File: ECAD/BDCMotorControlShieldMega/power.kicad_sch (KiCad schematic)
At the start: 23 parts, among them Q1 Q_PMOS, Q2 Q_PMOS, Q3 Q_NMOS, Q4 Q_NMOS, Q5 Q_PNP, Q6 Q_PNP, U14 LMV331, U33 LM2776

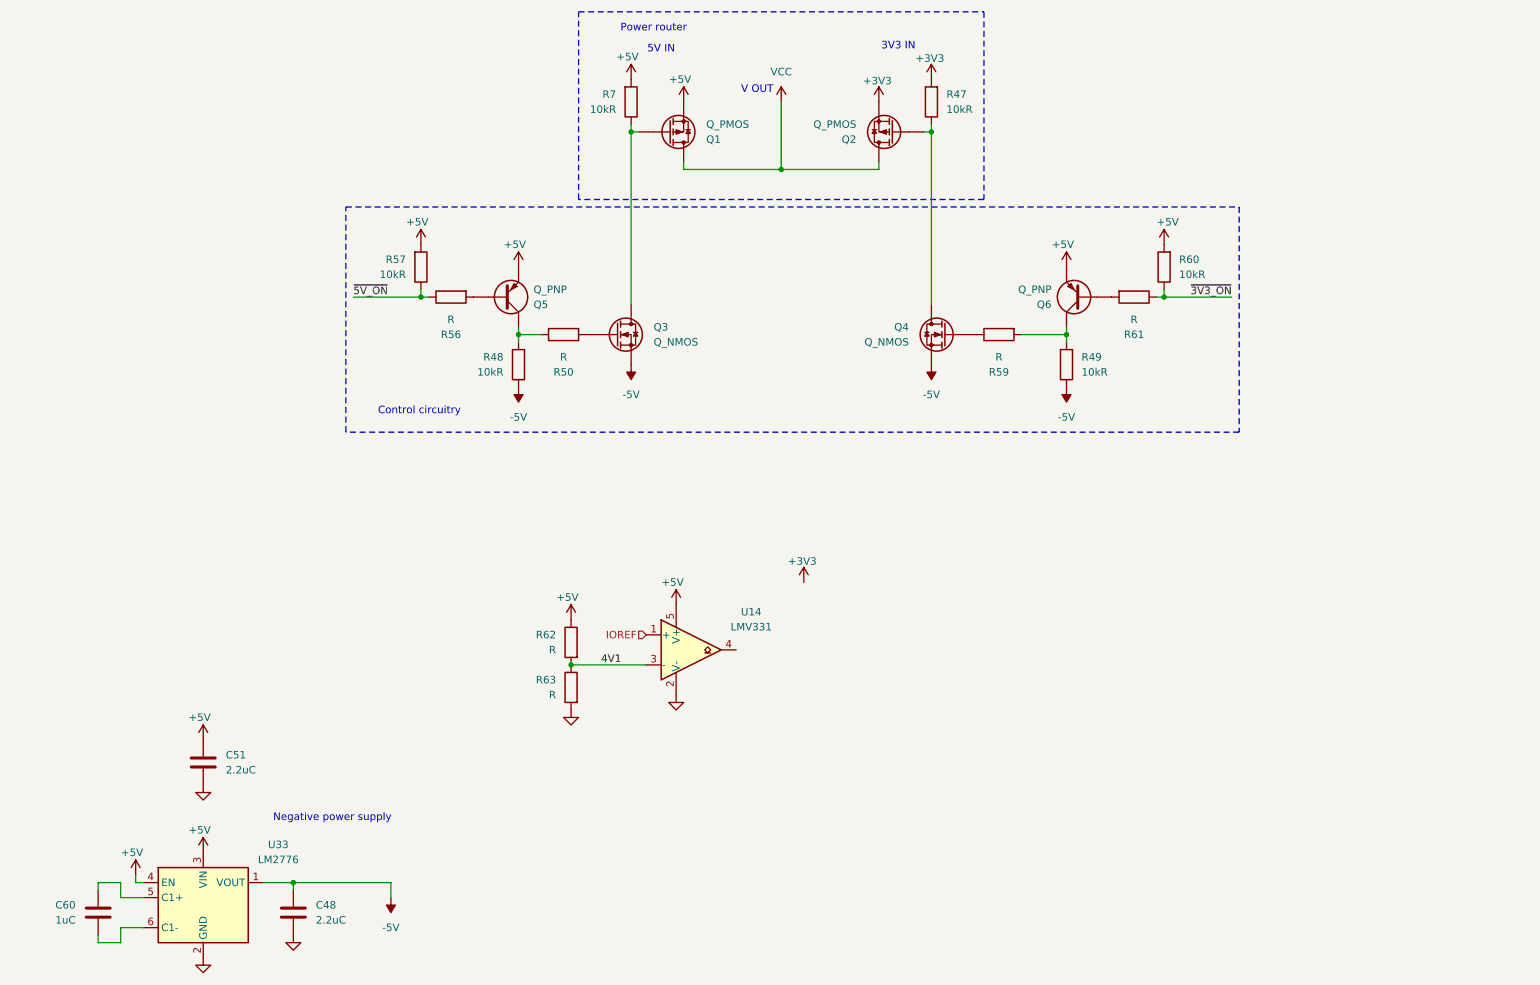
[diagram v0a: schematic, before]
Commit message: Update power.kicad_sch
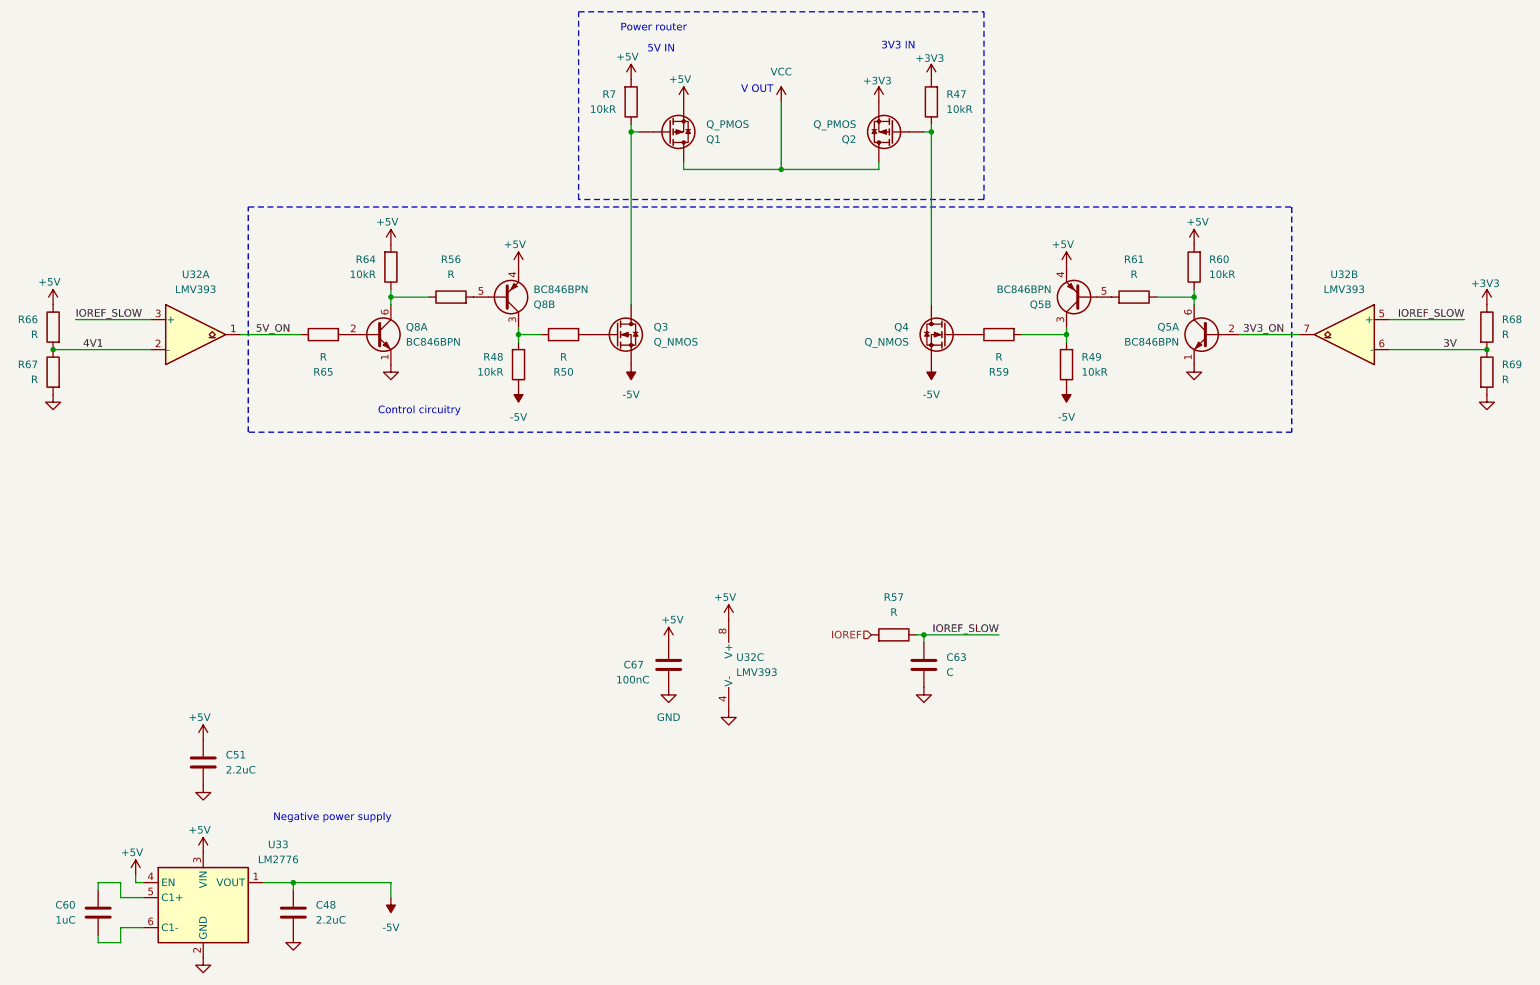
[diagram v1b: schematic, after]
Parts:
- removed Q5, Q6: Q_PNP, symbol Device:Q_PNP
- removed R62, R63: R, symbol Device:R
- removed U14: LMV331, symbol Comparator:LMV331
- added C63: C, symbol Device:C
- added C67: 100nC, Capacitor_SMD:C_0805_2012Metric, symbol Device:C
- added Q5, Q8: BC846BPN, Package_TO_SOT_SMD:SOT-363_SC-70-6, symbol Transistor_BJT:BC846BPN
- added R64: 10kR, Resistor_SMD:R_0805_2012Metric, symbol Device:R
- added R65, R66, R67, R68, R69: R, symbol Device:R
- added U32: LMV393, symbol Comparator:LMV393
- R57: value 10kR -> R; footprint Resistor_SMD:R_0805_2012Metric -> (none); MPN RC0805JR-0710KL -> (none); Status OK -> (none)
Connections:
- net +3V3: now also R68.1
- net +5V: now also C67.1, Q5.4 (E2), Q8.4 (E2), R64.2, R66.1, U32.8 (V+); no longer R57.2
- net 4V1: now also R66.2, R67.1, U32.2 (-)
- net GND: now also C63.2, C67.2, Q5.1 (E1), Q8.1 (E1), R67.2, R69.2, U32.4 (V-)
- net IOREF: now also R57.2
- net at R61.2: now also Q5.5 (B2)
- net at R49.2, R59.2: now also Q5.3 (C2)
- net at R56.2: now also Q8.5 (B2)
- net at R48.2, R50.1: now also Q8.3 (C2)
- net ~{3V3_ON}: no longer names the net of R60.1, R61.1
- net ~{3V3_ON}: now also Q5.6 (C1)
- net ~{5V_ON}: no longer names the net of R56.1
- net ~{5V_ON}: now also Q8.6 (C1), R64.1; no longer R57.1
- new net: Q8.2 (B1), R65.2
- new net 3V: R68.2, R69.1, U32.6 (-)
- new net 3V3_ON: Q5.2 (B1), U32.7
- new net 5V_ON: R65.1, U32.1
- new net IOREF_SLOW: C63.1, R57.1, U32.3 (+), U32.5 (+)
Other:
- moved on the sheet: R60

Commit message: Progressed ECAD.
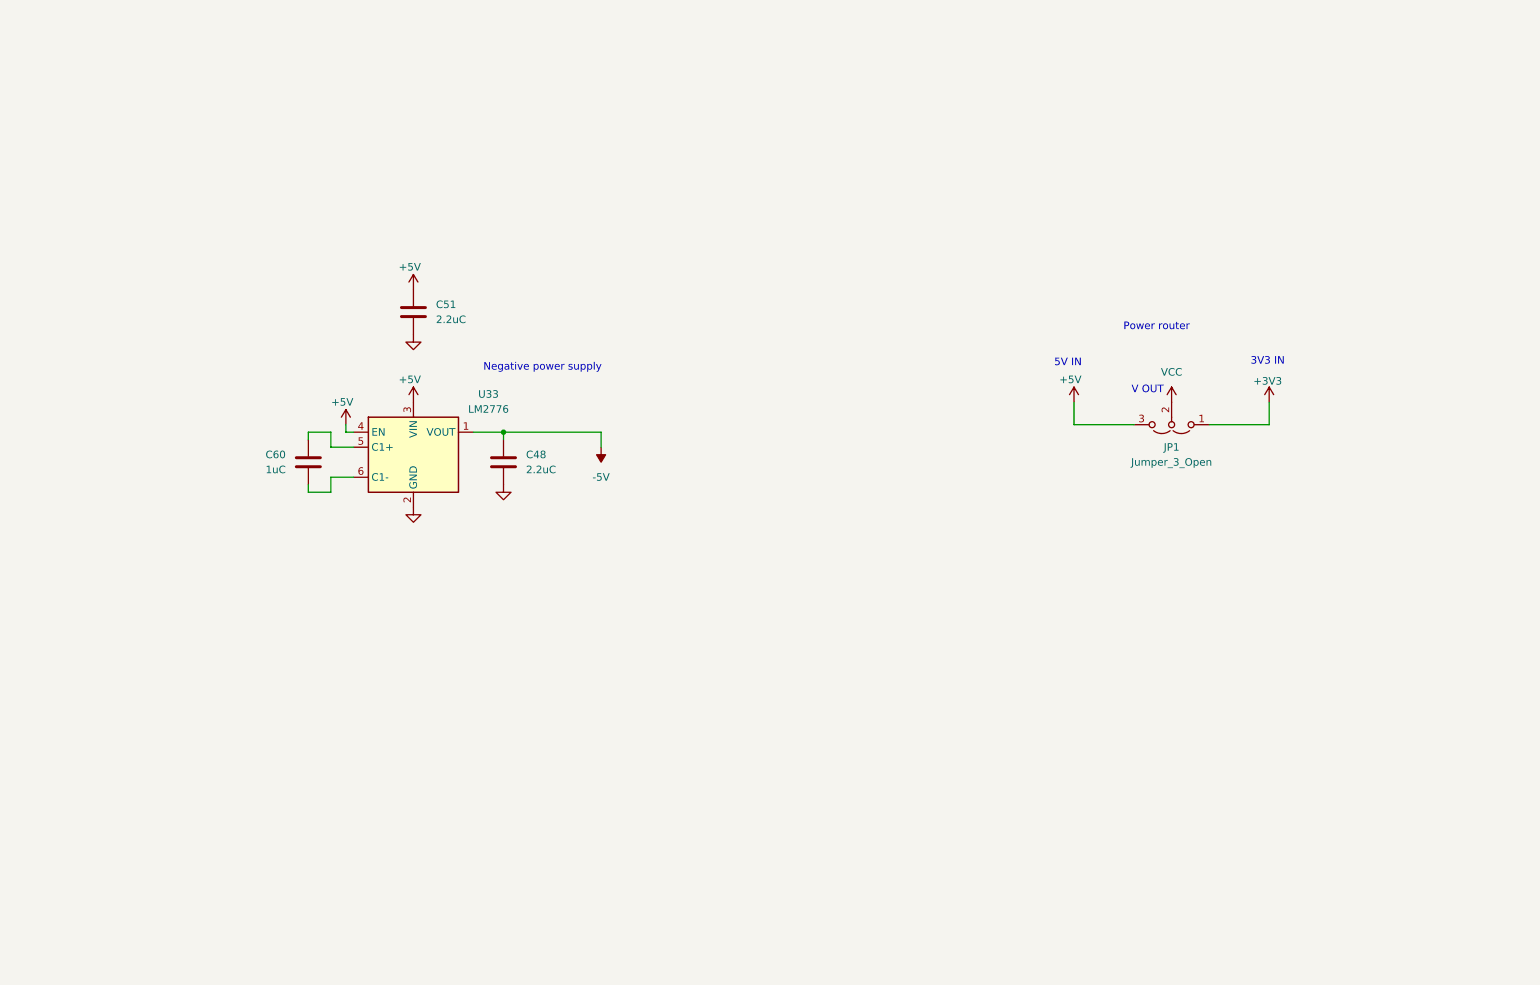
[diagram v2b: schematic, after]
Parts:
- removed C63: C, symbol Device:C
- removed C67: 100nC, Capacitor_SMD:C_0805_2012Metric, symbol Device:C
- removed Q1, Q2: Q_PMOS, symbol Device:Q_PMOS
- removed Q3, Q4: Q_NMOS, symbol Device:Q_NMOS
- removed Q5, Q8: BC846BPN, Package_TO_SOT_SMD:SOT-363_SC-70-6, symbol Transistor_BJT:BC846BPN
- removed R47, R48, R49, R60, R64, R7: 10kR, Resistor_SMD:R_0805_2012Metric, symbol Device:R
- removed R50, R56, R57, R59, R61, R65, R66, R67, R68, R69: R, symbol Device:R
- removed U32: LMV393, symbol Comparator:LMV393
- added JP1: Jumper_3_Open, Connector_PinHeader_2.54mm:PinHeader_1x03_P2.54mm_Vertical, symbol Jumper:Jumper_3_Open
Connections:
- net +3V3: now also JP1.1 (A)
- net +5V: now also JP1.3 (B)
- net VCC: now also JP1.2 (C)
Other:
- note removed: "Control circuitry"
- moved on the sheet: C48, C51, C60, U33

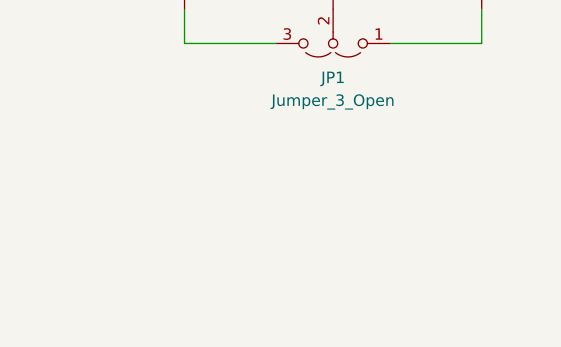
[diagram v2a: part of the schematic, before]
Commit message: Progressed ECAD.
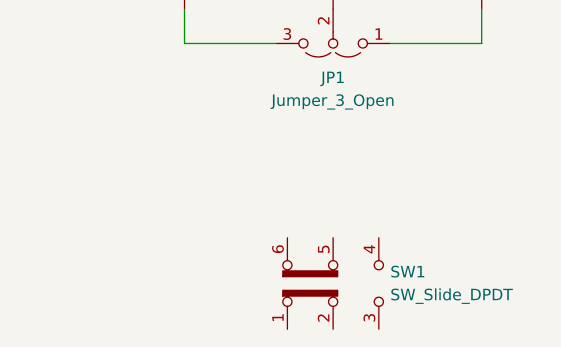
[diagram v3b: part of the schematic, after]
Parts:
- added SW1: SW_Slide_DPDT, Button_Switch_SMD:SW_SPDT_CK_JS102011SAQN, symbol Switch:SW_Slide_DPDT
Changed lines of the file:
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@@
+	)
+	(symbol
+		(lib_id "Switch:SW_Slide_DPDT")
+		(at 212.09 123.19 90)
+		(unit 1)
+		(exclude_from_sim no)
+		(in_bom yes)
+		(on_board yes)
+		(dnp no)
+		(fields_autoplaced yes)
+		(property "Reference" "SW1"
+			(at 218.44 121.9199 90)
+			(effects
+				(font
+					(size 1.27 1.27)
+				)
+				(justify right)
+			)
+		)
+		(property "Value" "SW_Slide_DPDT"
+			(at 218.44 124.4599 90)
+			(effects
+				(font
+					(size 1.27 1.27)
+				)
+				(justify right)
+			)
+		)
+		(property "Footprint" "Button_Switch_SMD:SW_SPDT_CK_JS102011SAQN"
+			(at 207.01 109.22 0)
+			(effects
+				(font
+					(size 1.27 1.27)
+				)
+				(hide yes)
+			)
+		)
+		(property "Datasheet" "~"
+			(at 212.09 123.19 0)
+			(effects
+				(font
+					(size 1.27 1.27)
+				)
+				(hide yes)
+			)
+		)
+		(property "Description" "Slide Switch, dual pole double throw"
+			(at 212.09 123.19 0)
+			(effects
+				(font
+					(size 1.27 1.27)
+				)
+				(hide yes)
+			)
+		)
+		(pin "3"
+		)
+		(pin "4"
+		)
+		(pin "6"
+		)
+		(pin "1"
+		)
+		(pin "2"
+		)
+		(pin "5"
+		)
+		(instances
+			(project ""
+				(path "/e63e39d7-6ac0-4ffd-8aa3-1841a4541b55/ba083037-3551-4343-972e-1d3a68128020"
+					(reference "SW1")
+					(unit 1)
+				)
+			)
+		)
 	)
 	(symbol

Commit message: Progressed ECAD.
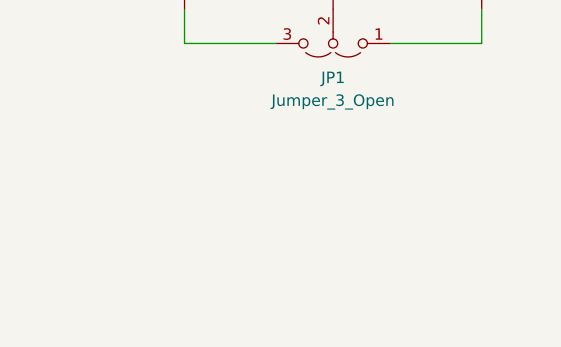
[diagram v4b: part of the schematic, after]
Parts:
- removed SW1: SW_Slide_DPDT, Button_Switch_SMD:SW_SPDT_CK_JS102011SAQN, symbol Switch:SW_Slide_DPDT
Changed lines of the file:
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@@
-	)
-	(symbol
-		(lib_id "Switch:SW_Slide_DPDT")
-		(at 212.09 123.19 90)
-		(unit 1)
-		(exclude_from_sim no)
-		(in_bom yes)
-		(on_board yes)
-		(dnp no)
-		(fields_autoplaced yes)
-		(property "Reference" "SW1"
-			(at 218.44 121.9199 90)
-			(effects
-				(font
-					(size 1.27 1.27)
-				)
-				(justify right)
-			)
-		)
-		(property "Value" "SW_Slide_DPDT"
-			(at 218.44 124.4599 90)
-			(effects
-				(font
-					(size 1.27 1.27)
-				)
-				(justify right)
-			)
-		)
-		(property "Footprint" "Button_Switch_SMD:SW_SPDT_CK_JS102011SAQN"
-			(at 207.01 109.22 0)
-			(effects
-				(font
-					(size 1.27 1.27)
-				)
-				(hide yes)
-			)
-		)
-		(property "Datasheet" "~"
-			(at 212.09 123.19 0)
-			(effects
-				(font
-					(size 1.27 1.27)
-				)
-				(hide yes)
-			)
-		)
-		(property "Description" "Slide Switch, dual pole double throw"
-			(at 212.09 123.19 0)
-			(effects
-				(font
-					(size 1.27 1.27)
-				)
-				(hide yes)
-			)
-		)
-		(pin "3"
-		)
-		(pin "4"
-		)
-		(pin "6"
-		)
-		(pin "1"
-		)
-		(pin "2"
-		)
-		(pin "5"
-		)
-		(instances
-			(project ""
-				(path "/e63e39d7-6ac0-4ffd-8aa3-1841a4541b55/ba083037-3551-4343-972e-1d3a68128020"
-					(reference "SW1")
-					(unit 1)
-				)
-			)
-		)
 	)
 	(symbol
